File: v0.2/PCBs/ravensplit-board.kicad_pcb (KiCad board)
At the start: 2 copper layers, 126.6 x 113.9 mm, 48 parts

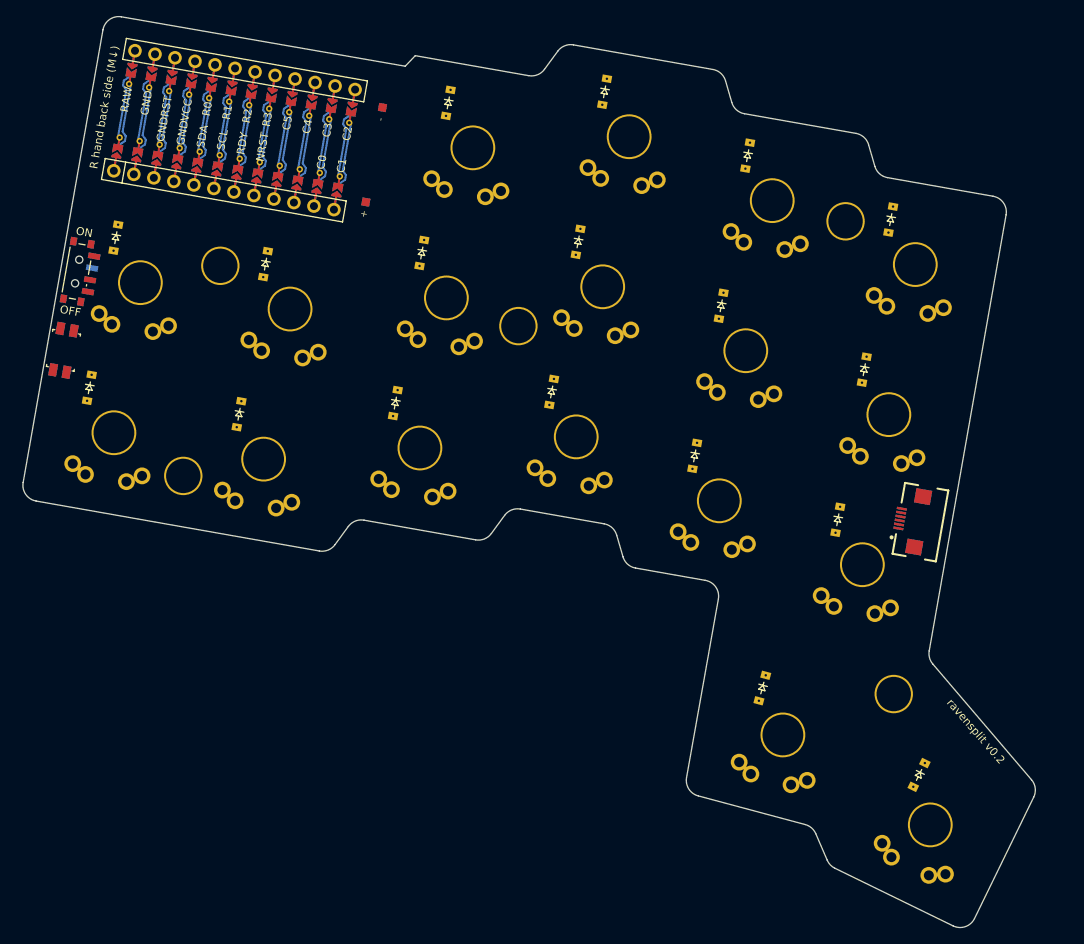
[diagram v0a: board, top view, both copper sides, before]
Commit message: Add routed PCBs and Gerbers
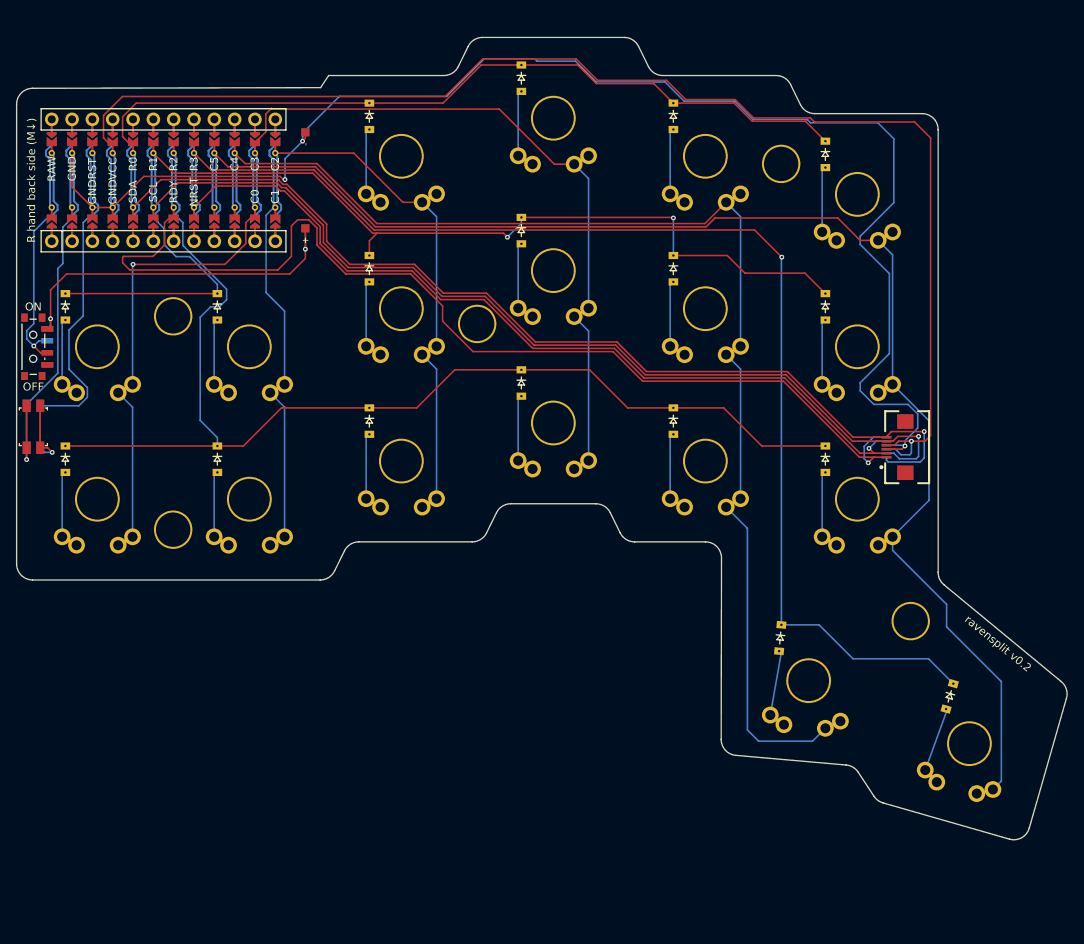
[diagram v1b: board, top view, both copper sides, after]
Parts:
- moved D16 11.5 mm to (170.0, 81.1), turned to -90 degrees
- moved S16 11.4 mm to (174.0, 86.1), turned to 0 degrees
- moved S17 11.3 mm to (188.1, 154.7), turned to -16 degrees
- moved MCU1 11.0 mm to (86.0, 84.3), turned to 90 degrees
- moved PWR1 10.9 mm to (71.0, 105.1), turned to 180 degrees
- moved MH1 10.8 mm to (164.5, 82.2), turned to 0 degrees
- moved D2 10.7 mm to (75.0, 100.1), turned to -90 degrees
- moved D10 10.5 mm to (132.0, 71.5), turned to -90 degrees
- moved D17 10.5 mm to (185.6, 148.8), turned to -106 degrees
- moved D13 10.5 mm to (151.0, 76.3), turned to -90 degrees
- moved RST1 10.3 mm to (71.0, 115.1), turned to 90 degrees
- moved PAD2 10.1 mm to (105.0, 78.3), turned to 90 degrees
- moved S13 10.0 mm to (155.0, 81.3), turned to 0 degrees
- moved D7 10.0 mm to (113.0, 76.3), turned to -90 degrees
- moved S10 9.75 mm to (136.0, 76.5), turned to 0 degrees
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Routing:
- net (no net): track 337.7 -> 39.4 mm
- net GND: track 0.00 -> 246.5 mm, vias 0 -> 4
- net C5: track 0.00 -> 177.5 mm
- net VCC: track 0.00 -> 172.6 mm, vias 0 -> 1
- net R3: track 0.00 -> 159.2 mm, vias 0 -> 1
- net C4: track 0.00 -> 153.5 mm
- net R2: track 0.00 -> 147.2 mm
- net RDY: track 0.00 -> 142.4 mm, vias 0 -> 1
- net R1: track 0.00 -> 142.4 mm, vias 0 -> 2
- net SDA: track 0.00 -> 133.9 mm, vias 0 -> 1
- net SCL: track 0.00 -> 128.6 mm, vias 0 -> 1
- net NRST: track 0.00 -> 116.0 mm, vias 0 -> 1
- net R0: track 0.00 -> 108.4 mm
- net C3: track 0.00 -> 93.2 mm
- net C2: track 0.00 -> 68.2 mm
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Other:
- board size 126.6 x 113.9 mm -> 131.3 x 100.3 mm
